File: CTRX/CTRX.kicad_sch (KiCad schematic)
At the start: 33 parts, among them J1 USB_B_Micro, J2 SMA_CONNECTOR, J3 Conn_02x05_Odd_Even, U1 nRF52820-QDxx, U2 NRF21540-QDAA-R7, U3 USBLC6-2SC6, U4 ME6211C33M5, Y1 32MHz

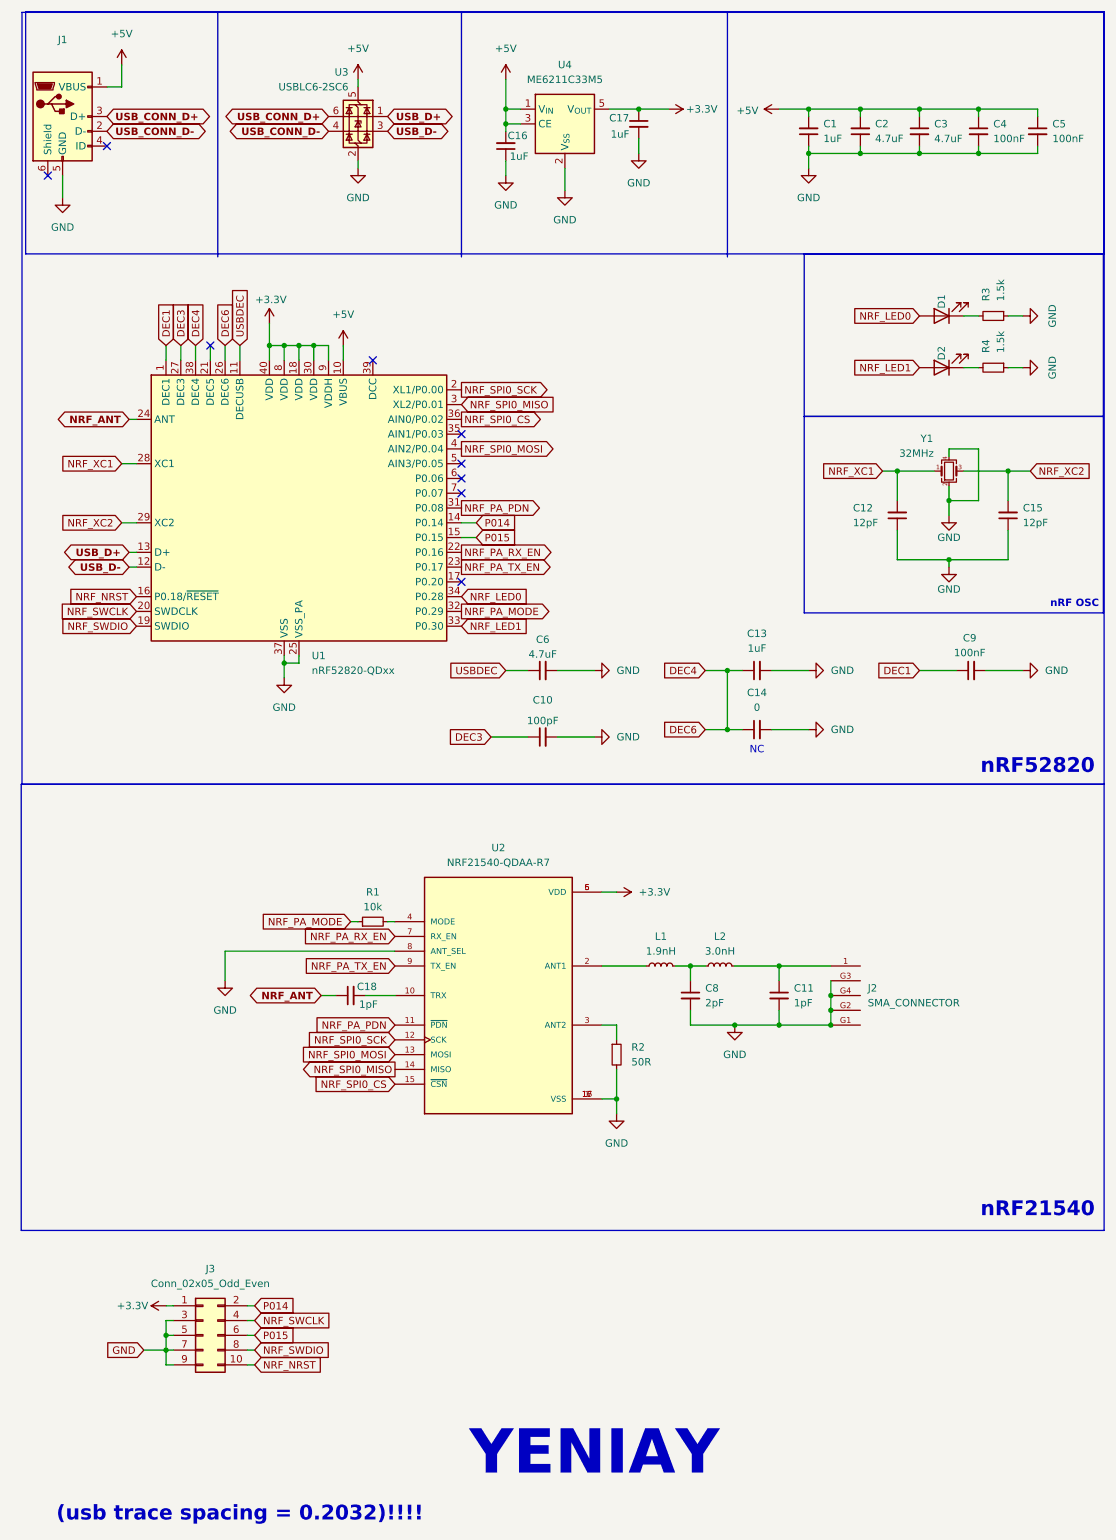
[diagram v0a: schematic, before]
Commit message: schematic updated
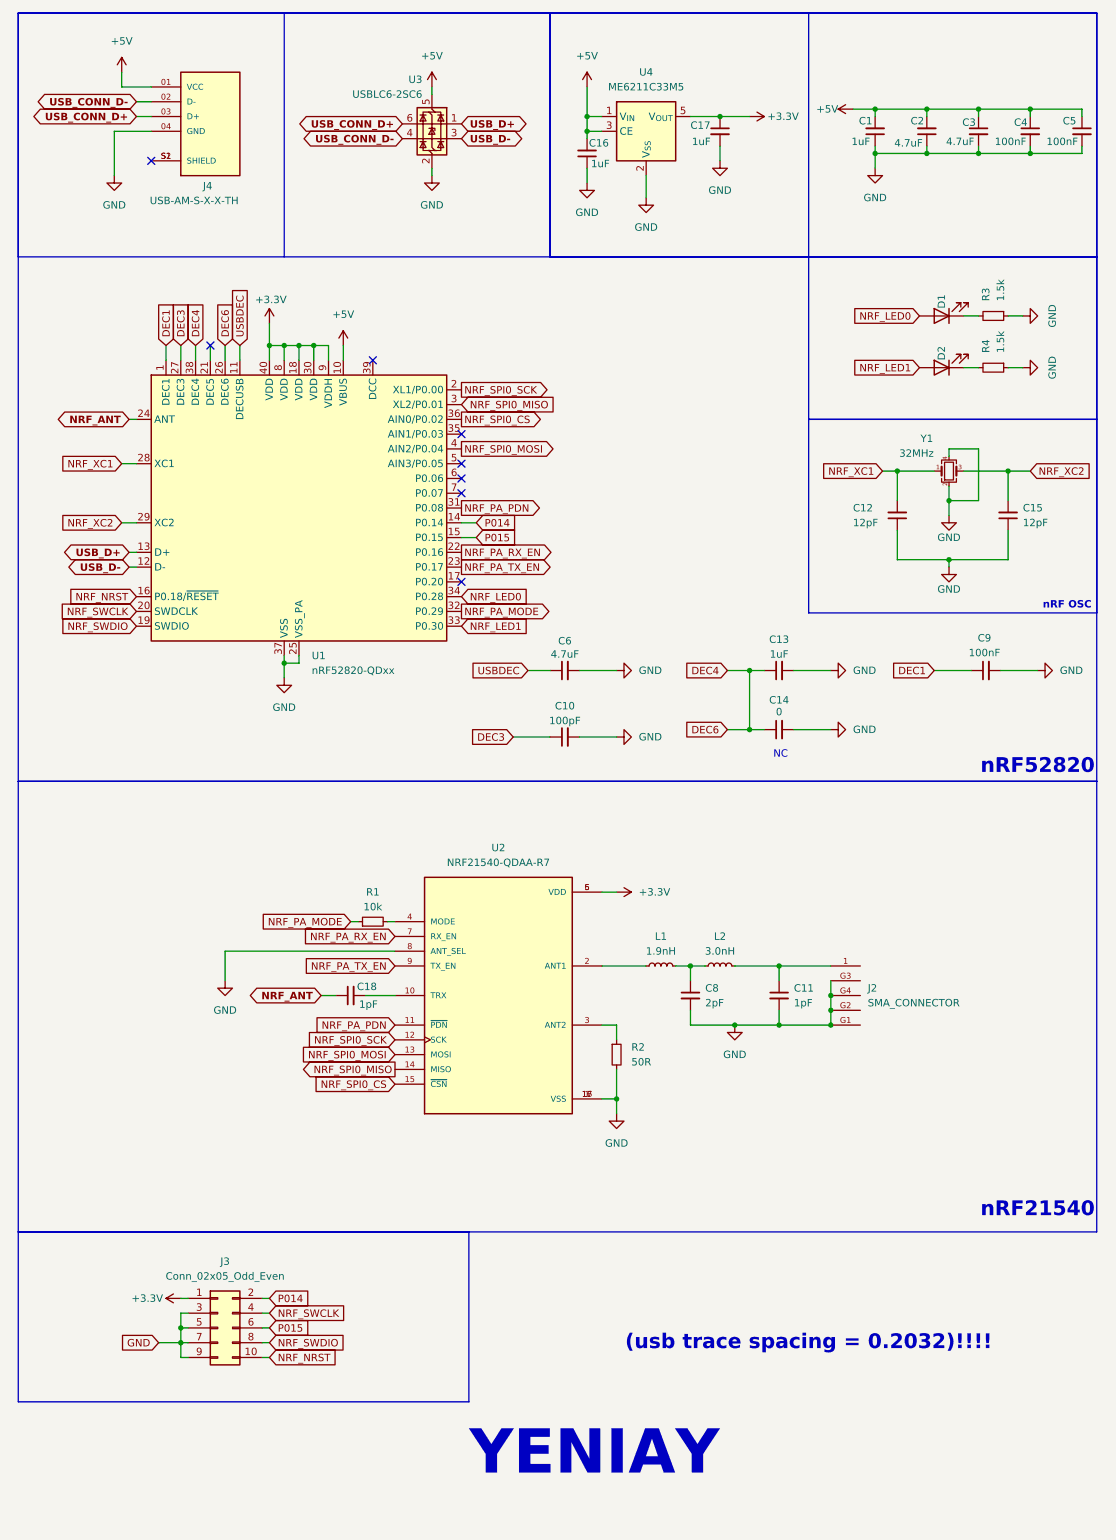
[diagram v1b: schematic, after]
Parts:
- removed J1: USB_B_Micro, symbol Connector:USB_B_Micro
- added J4: USB-AM-S-X-X-TH, USB-AM-S-X-X-TH:SAMTEC_USB-AM-S-X-X-TH, symbol USB-AM-S-X-X-TH:USB-AM-S-X-X-TH
- C16, C17: footprint (none) -> Capacitor_SMD:C_0402_1005Metric
- C3: footprint Capacitor_SMD:C_0201_0603Metric -> Capacitor_SMD:C_0603_1608Metric
- J3: footprint (none) -> Connector_IDC:IDC-Header_2x05_P2.54mm_Vertical
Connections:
- net +5V: now also J4.01 (VCC)
- net GND: now also J4.04 (GND)
- net USB_CONN_D+: now also J4.03 (D+)
- net USB_CONN_D-: now also J4.02 (D-)
- new net: J4.S1 (SHIELD), J4.S2 (SHIELD)
- no-connect marks 9 -> 8
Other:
- moved on the sheet: C1, C10, C13, C14, C16, C17, C2, C3, C4, C5, C6, C9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
